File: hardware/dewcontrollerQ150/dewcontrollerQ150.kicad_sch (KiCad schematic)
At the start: 13 parts, among them J1 12V Power, J2 Dew Heater, J3 SHT45 Sensor, Q1 FQP 30N06L, U1 XIAO-ESP32-C3-DIP, U2 Buck_12V_5V

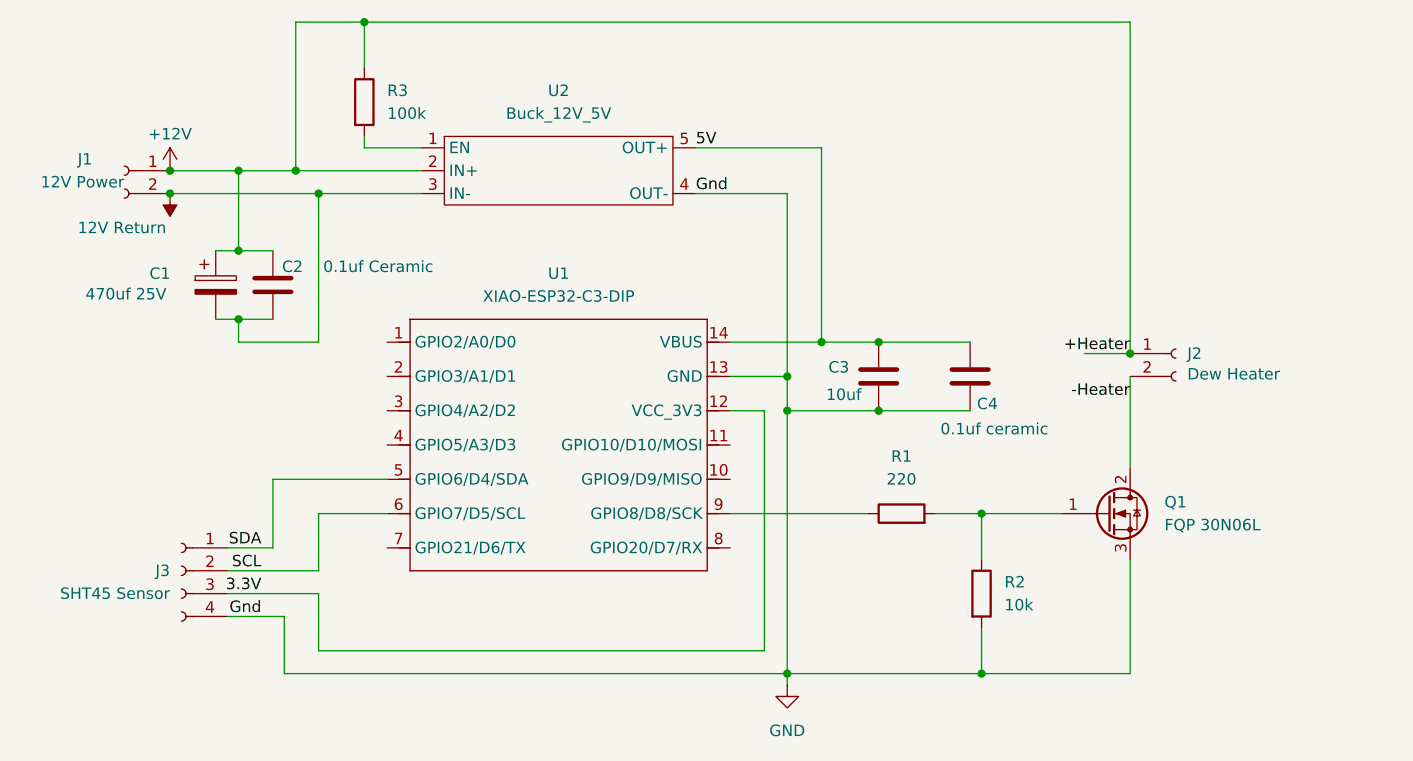
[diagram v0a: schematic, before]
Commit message: V0.51 updated KiCAD schematic with S3
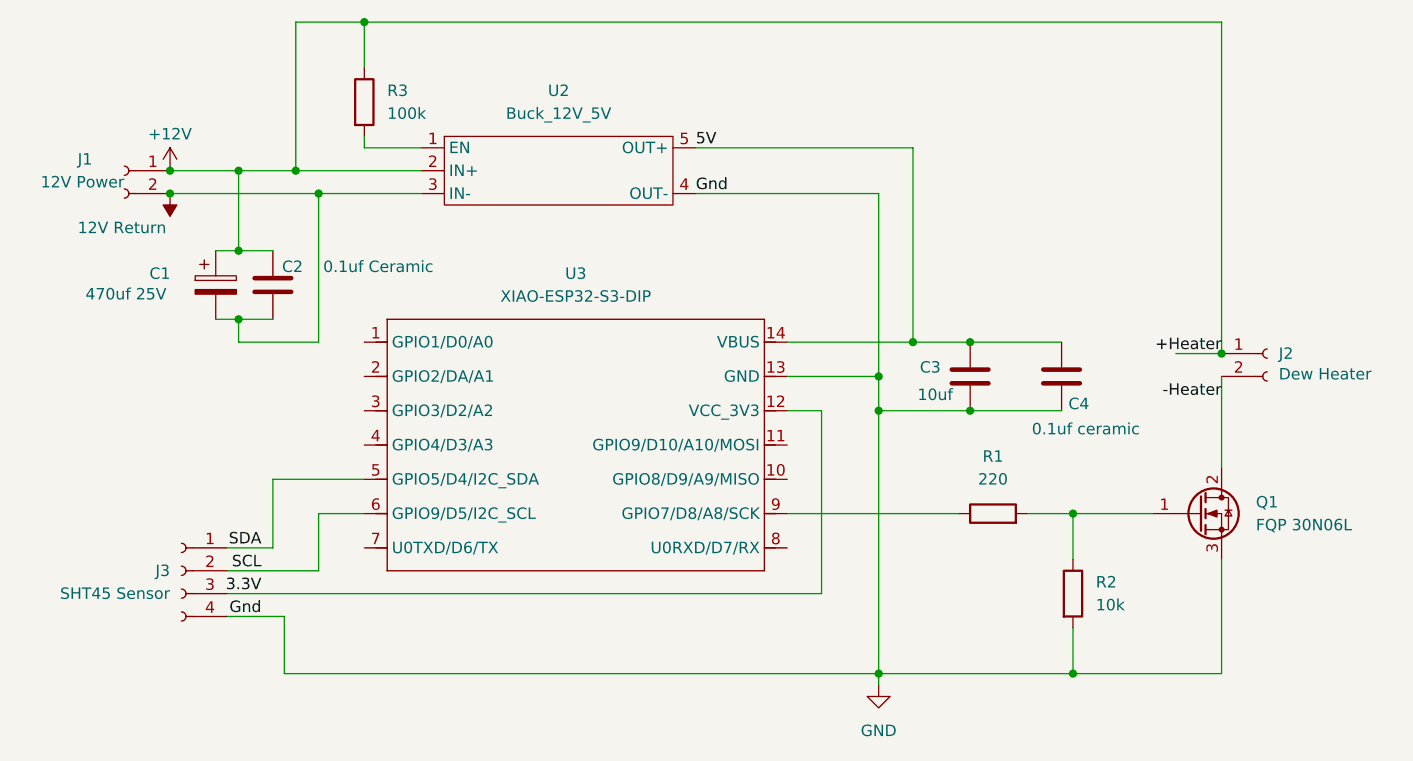
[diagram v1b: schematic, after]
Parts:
- removed U1: XIAO-ESP32-C3-DIP, Module:MOUDLE14P-XIAO-DIP-SMD, symbol Seeed_Studio_XIAO_Series:XIAO-ESP32-C3-DIP
- added U3: XIAO-ESP32-S3-DIP, RF_Module:MCU_Seeed_ESP32C3, symbol Seeed_Studio_XIAO_Series:XIAO-ESP32-S3-DIP
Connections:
- net 3.3V: now also U3.12 (VCC_3V3)
- net 5V: now also U3.14 (VBUS)
- net GND: now also U3.13 (GND)
- net SCL: now also U3.6 (GPIO9/D5/I2C_SCL)
- net SDA: now also U3.5 (GPIO5/D4/I2C_SDA)
- net at R1.1: now also U3.9 (GPIO7/D8/A8/SCK)
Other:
- moved on the sheet: C3, C4, J2, Q1, R1, R2
